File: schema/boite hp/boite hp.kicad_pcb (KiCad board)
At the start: 2 copper layers, 24 parts, among them J1 IN-, J2 IN+, J3 B+, J4 B-, J5 Bracelet+, J6 Bracelet-, U1 IP2312, U2 IP2312, U3 ESP-32D, U4 LDO 3v3, U5 PCM5102A, U6 PAM8403, U7 HP

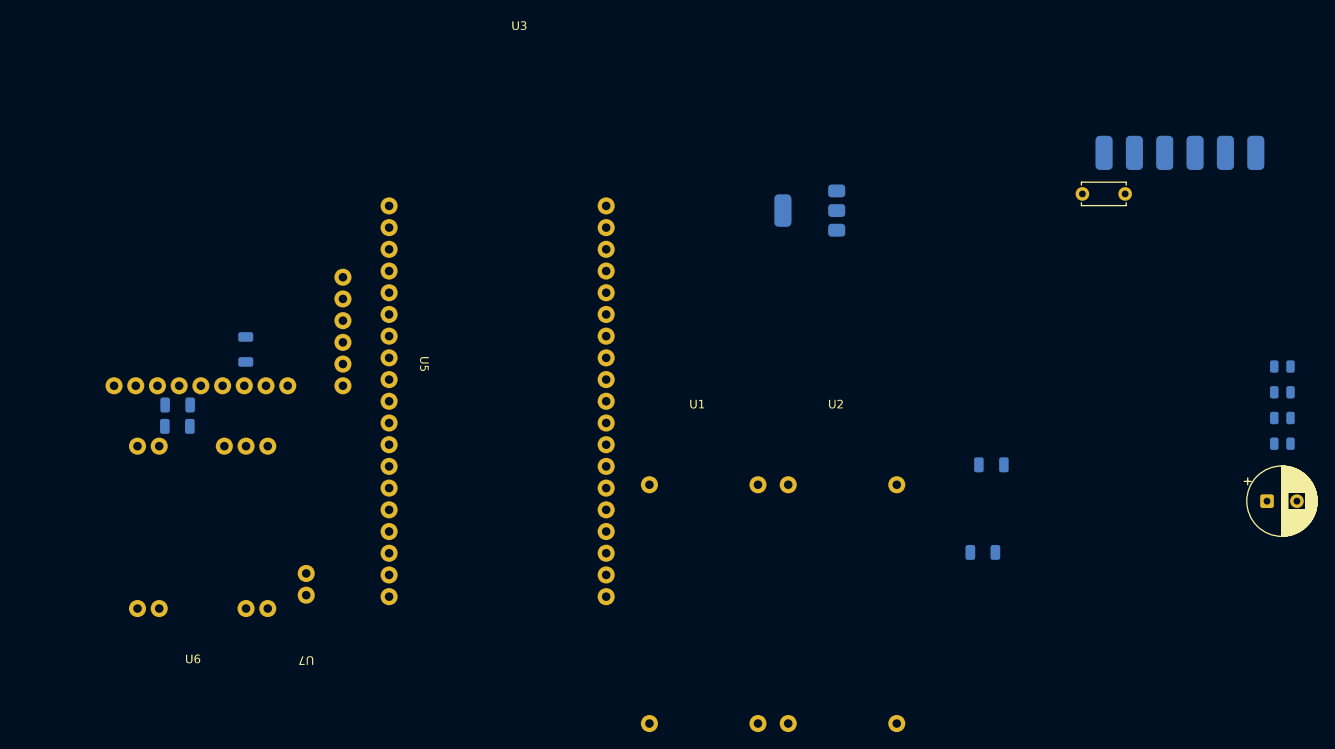
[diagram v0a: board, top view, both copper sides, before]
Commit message: Update Architecture db
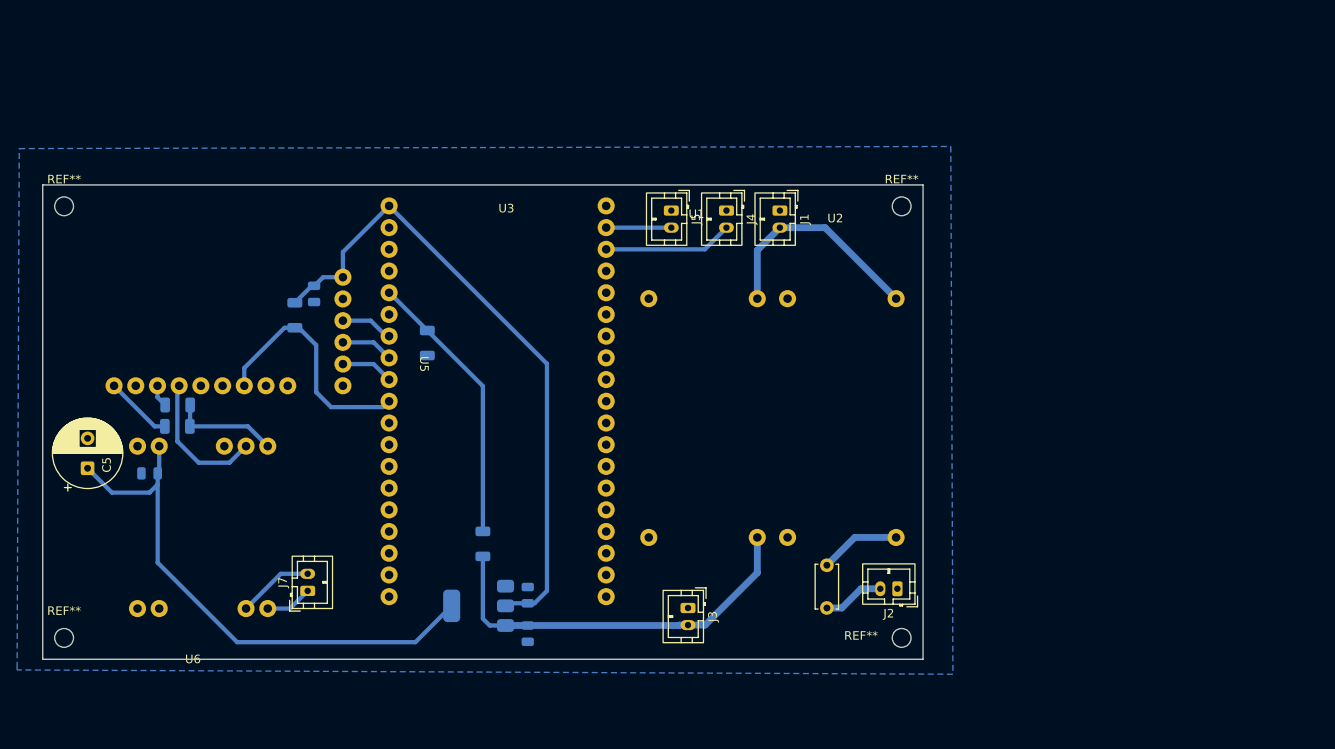
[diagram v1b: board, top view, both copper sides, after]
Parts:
- removed J6: Bracelet-, Connector_Wire:SolderWirePad_1x01_SMD_2x4mm
- removed U7: HP, Library_Perso:Connector_boxed_2.54_1x02
- added J7: HP, Connector_JST:JST_PH_B2B-PH-K_1x02_P2.00mm_Vertical, F.Cu at (98.5, 114.2)
- added REF**: MountingHole_2.2mm_M2, MountingHole:MountingHole_2.2mm_M2, F.Cu at (168.0, 69.2)
- added REF**: MountingHole_2.2mm_M2, MountingHole:MountingHole_2.2mm_M2, F.Cu at (168.0, 119.8)
- added REF**: MountingHole_2.2mm_M2, MountingHole:MountingHole_2.2mm_M2, F.Cu at (70.0, 119.8)
- added REF**: MountingHole_2.2mm_M2, MountingHole:MountingHole_2.2mm_M2, F.Cu at (70.0, 69.2)
- J1: value IN- -> IN; footprint Connector_Wire:SolderWirePad_1x01_SMD_2x4mm -> Connector_JST:JST_PH_B2B-PH-K_1x02_P2.00mm_Vertical; moved to F.Cu
- J2: value IN+ -> Bracelet; footprint Connector_Wire:SolderWirePad_1x01_SMD_2x4mm -> Connector_JST:JST_PH_B2B-PH-K_1x02_P2.00mm_Vertical; moved to F.Cu
- J3: value B+ -> Battery; footprint Connector_Wire:SolderWirePad_1x01_SMD_2x4mm -> Connector_JST:JST_PH_B2B-PH-K_1x02_P2.00mm_Vertical; moved to F.Cu
- J4: value B- -> res1; footprint Connector_Wire:SolderWirePad_1x01_SMD_2x4mm -> Connector_JST:JST_PH_B2B-PH-K_1x02_P2.00mm_Vertical; moved to F.Cu
- J5: value Bracelet+ -> res2; footprint Connector_Wire:SolderWirePad_1x01_SMD_2x4mm -> Connector_JST:JST_PH_B2B-PH-K_1x02_P2.00mm_Vertical; moved to F.Cu
- moved C5 138.1 mm to (72.8, 99.9), turned to 90 degrees
- moved C4 132.6 mm to (80.0, 100.5)
- moved C3 114.2 mm to (99.2, 79.5), turned to -90 degrees
- moved C2 92.7 mm to (124.2, 119.2), turned to -90 degrees
- moved C1 92.3 mm to (124.2, 114.8), turned to 90 degrees
- moved J3 79.7 mm to (143.0, 116.2), turned to -90 degrees
- moved R2 69.5 mm to (112.5, 85.2), turned to 90 degrees
- moved J2 63.8 mm to (167.5, 114.0)
- moved U4 60.3 mm to (118.5, 116.0)
- moved R1 60.2 mm to (119.0, 108.8), turned to 90 degrees
- moved F1 56.9 mm to (159.2, 116.2), turned to 90 degrees
- moved J1 56.1 mm to (153.8, 69.8), turned to -90 degrees
- moved J5 54.6 mm to (141.1, 69.8), turned to -90 degrees
- moved J4 51.7 mm to (147.5, 69.8), turned to -90 degrees
- moved U1 21.8 mm to (143.5, 75.0)
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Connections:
- C2 pad 1: Net-(J3-Pin_1) -> Net-(J3-Pin_2)
- F1 pad 1: Net-(J5-Pin_1) -> Net-(J2-Pin_2)
- J2 pad 1: Net-(J2-Pin_1) -> GND
- J3 pad 1: Net-(J3-Pin_1) -> GND
- J5 pad 1: Net-(J5-Pin_1) -> GND
- R1 pad 1: Net-(J3-Pin_1) -> Net-(J3-Pin_2)
- U1 pad B+: Net-(J3-Pin_1) -> Net-(J3-Pin_2)
- U1 pad IN+: Net-(J2-Pin_1) -> Net-(J1-Pin_2)
- U2 pad IN+: Net-(J2-Pin_1) -> Net-(J1-Pin_2)
- U3 pad 22: unconnected-(U3-IO22-Pad22) -> Net-(J4-Pin_2)
- U3 pad 23: unconnected-(U3-IO23-Pad23) -> Net-(J5-Pin_2)
- U4 pad 3: Net-(J3-Pin_1) -> Net-(J3-Pin_2)
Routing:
- net +3.3V: track 0.00 -> 139.2 mm
- net Net-(J3-Pin_2): track 0.00 -> 46.5 mm
- net Net-(U3-IO34): track 0.00 -> 32.5 mm
- net Net-(U3-IO26): track 0.00 -> 28.3 mm
- net Net-(J1-Pin_2): track 0.00 -> 26.4 mm
- net Net-(U5-PadAGND)_1: track 0.00 -> 16.5 mm
- net Net-(J4-Pin_2): track 0.00 -> 15.1 mm
- net Net-(R3-Pad2): track 0.00 -> 12.6 mm
- net Net-(F1-Pad2): track 0.00 -> 9.45 mm
- net Net-(J7-Pin_2): track 0.00 -> 8.89 mm
- net Net-(R4-Pad1): track 0.00 -> 7.91 mm
- net Net-(J5-Pin_2): track 0.00 -> 7.62 mm
- net Net-(J2-Pin_2): track 0.00 -> 7.18 mm
- net Net-(U3-IO32): track 0.00 -> 6.15 mm
- net Net-(U3-IO25): track 0.00 -> 6.15 mm
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- added copper zone on B.Cu, net GND
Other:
- board outline added: 103 x 55.5 mm
